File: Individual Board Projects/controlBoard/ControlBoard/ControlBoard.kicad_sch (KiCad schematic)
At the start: 12 parts, among them J1 USBCPD, J2 AudioJack3, J3 5x2.54mm+2xBus, U1 LMC6484, U2 LMC6484, U3 ESP32-C6-DEVKITC-1-N8

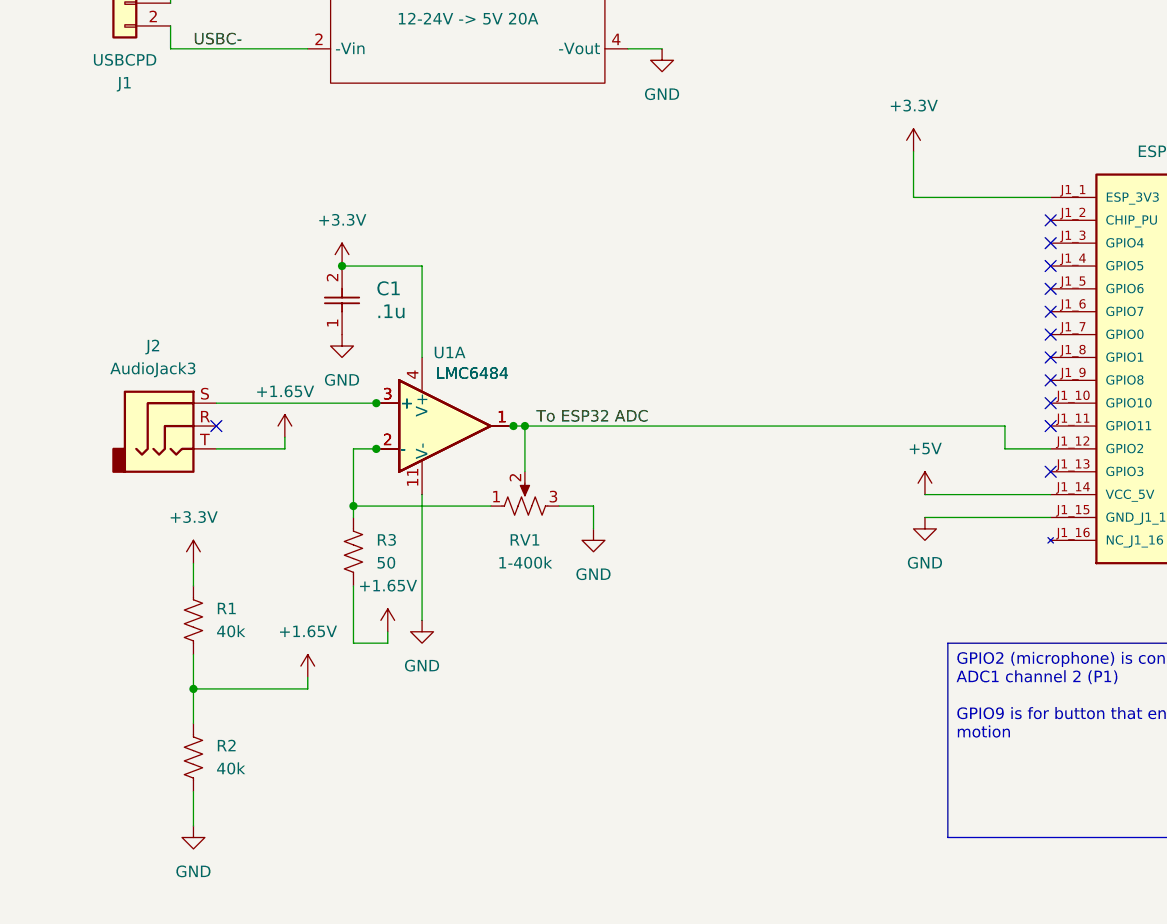
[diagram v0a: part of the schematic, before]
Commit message: Updated KiCad files
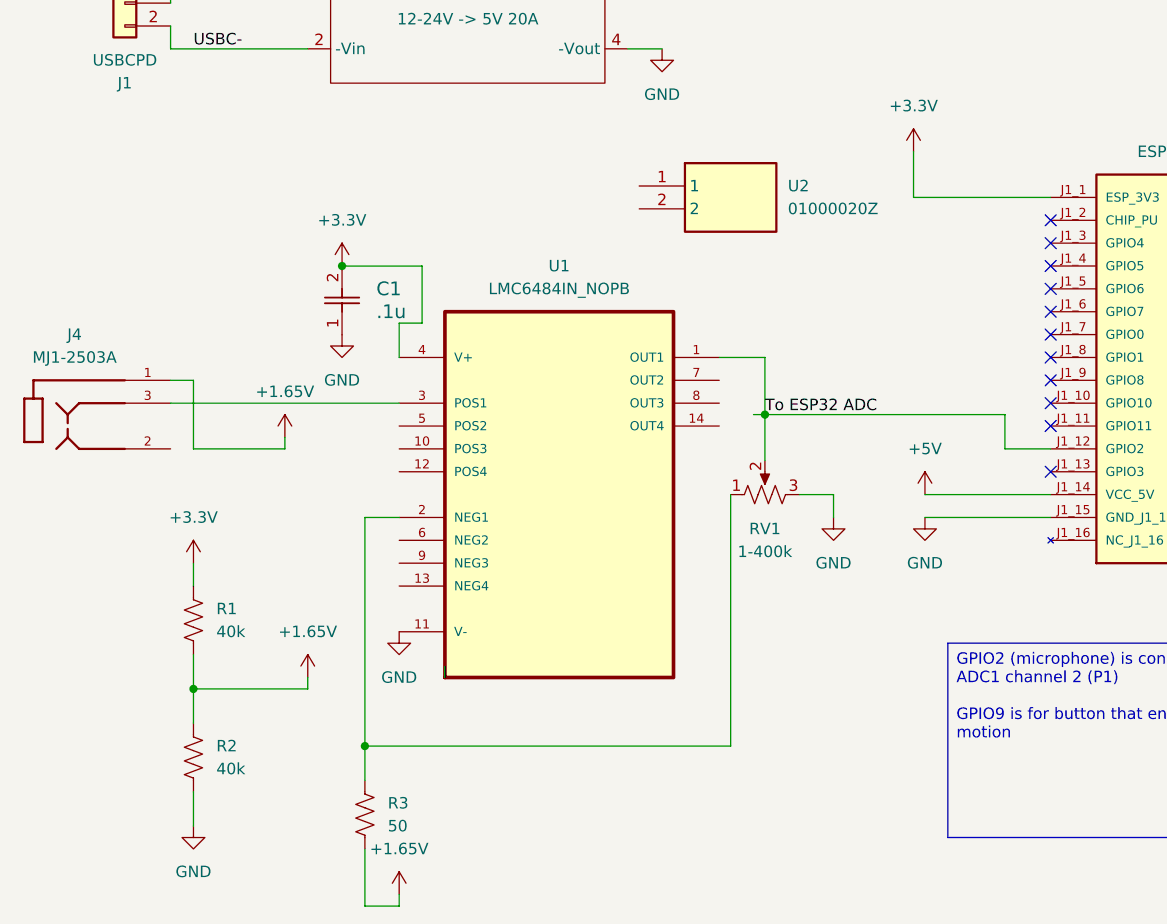
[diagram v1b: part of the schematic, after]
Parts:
- removed J2: AudioJack3, symbol Connector_Audio:AudioJack3
- removed U1, U2: LMC6484, Rose Actuator Library:DIP254P762X508-14, symbol Amplifier_Operational:LMC6484
- added J4: MJ1-2503A, Rose Actuator Library:SAMESKY_MJ1-2503A, symbol Rosethings:MJ1-2503A
- added U1: LMC6484IN_NOPB, Rose Actuator Library:DIP254P762X508-14, symbol LMC6484IN_NOPB:LMC6484IN_NOPB
- added U2: 01000020Z, 01000020Z, symbol Rosethings:01000020Z
- B1: footprint (none) -> BUCK_and_USBC:Buck-fourpins
- J1: footprint (none) -> BUCK_and_USBC:USBC-PD-Module-twopins
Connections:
- net +1.65V: now also J4.1
- net +3.3V: now also U1.4 (V+)
- net GND: now also U1.11 (V-)
- net To ESP32 ADC: now also U1.1 (OUT1)
- net at R3.1, RV1.1: now also U1.2 (NEG1)
- new net: J4.3, U1.3 (POS1)
- no-connect marks 22 -> 21
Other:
- moved on the sheet: R3, RV1
